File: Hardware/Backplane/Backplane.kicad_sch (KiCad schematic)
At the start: 3 parts, among them J101 10018784-10201TLF

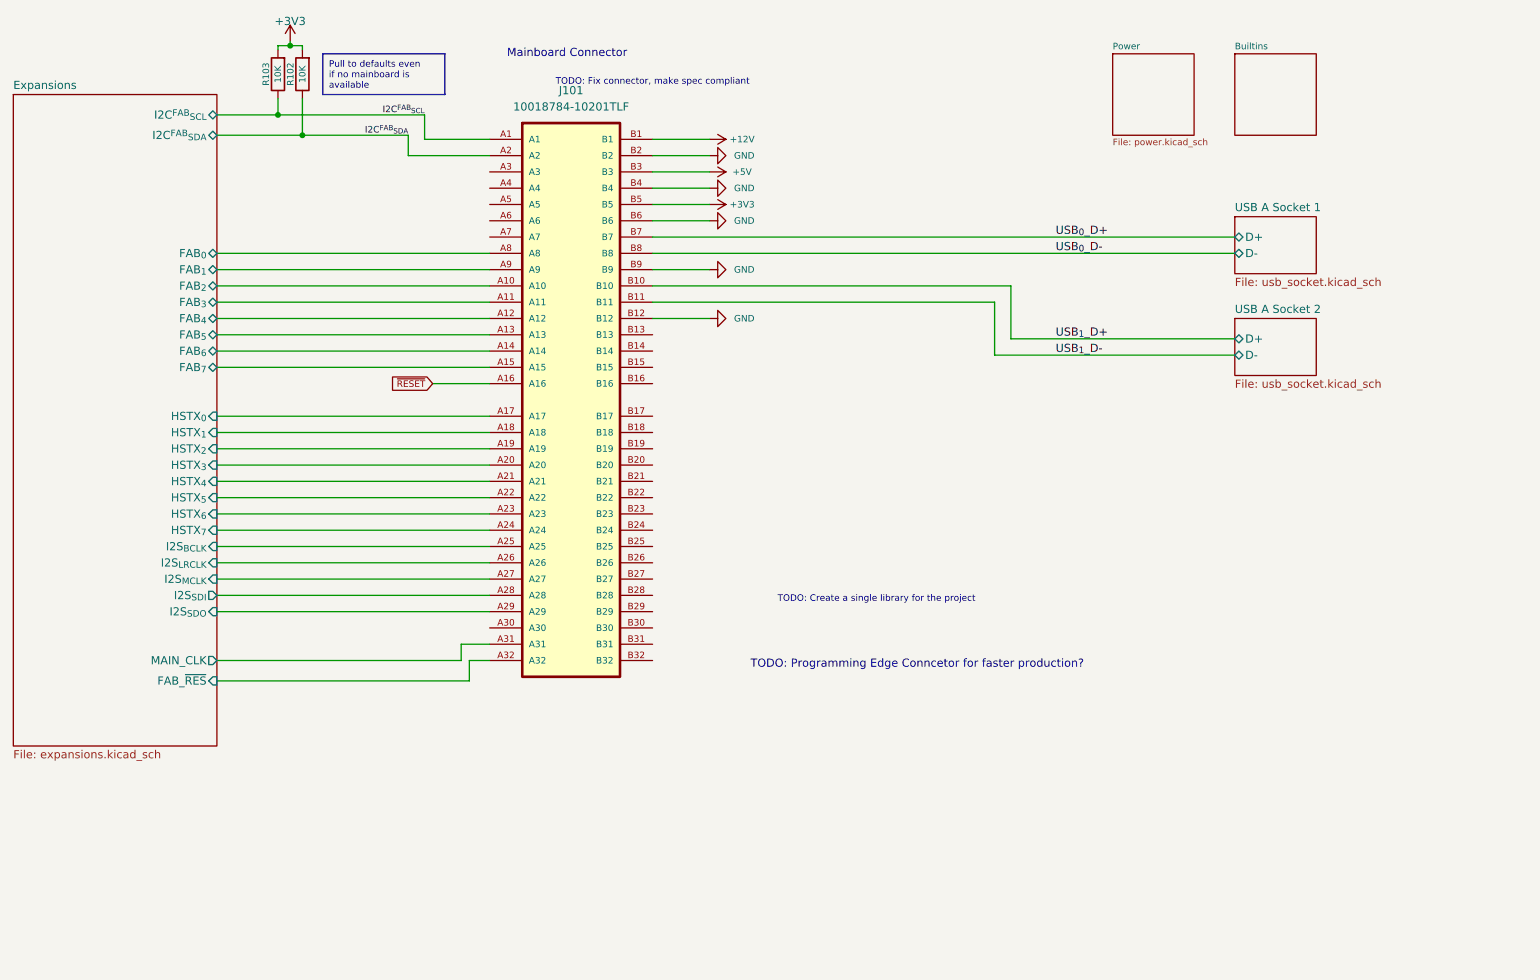
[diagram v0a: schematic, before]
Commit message: Further backplane PCB cleanup.
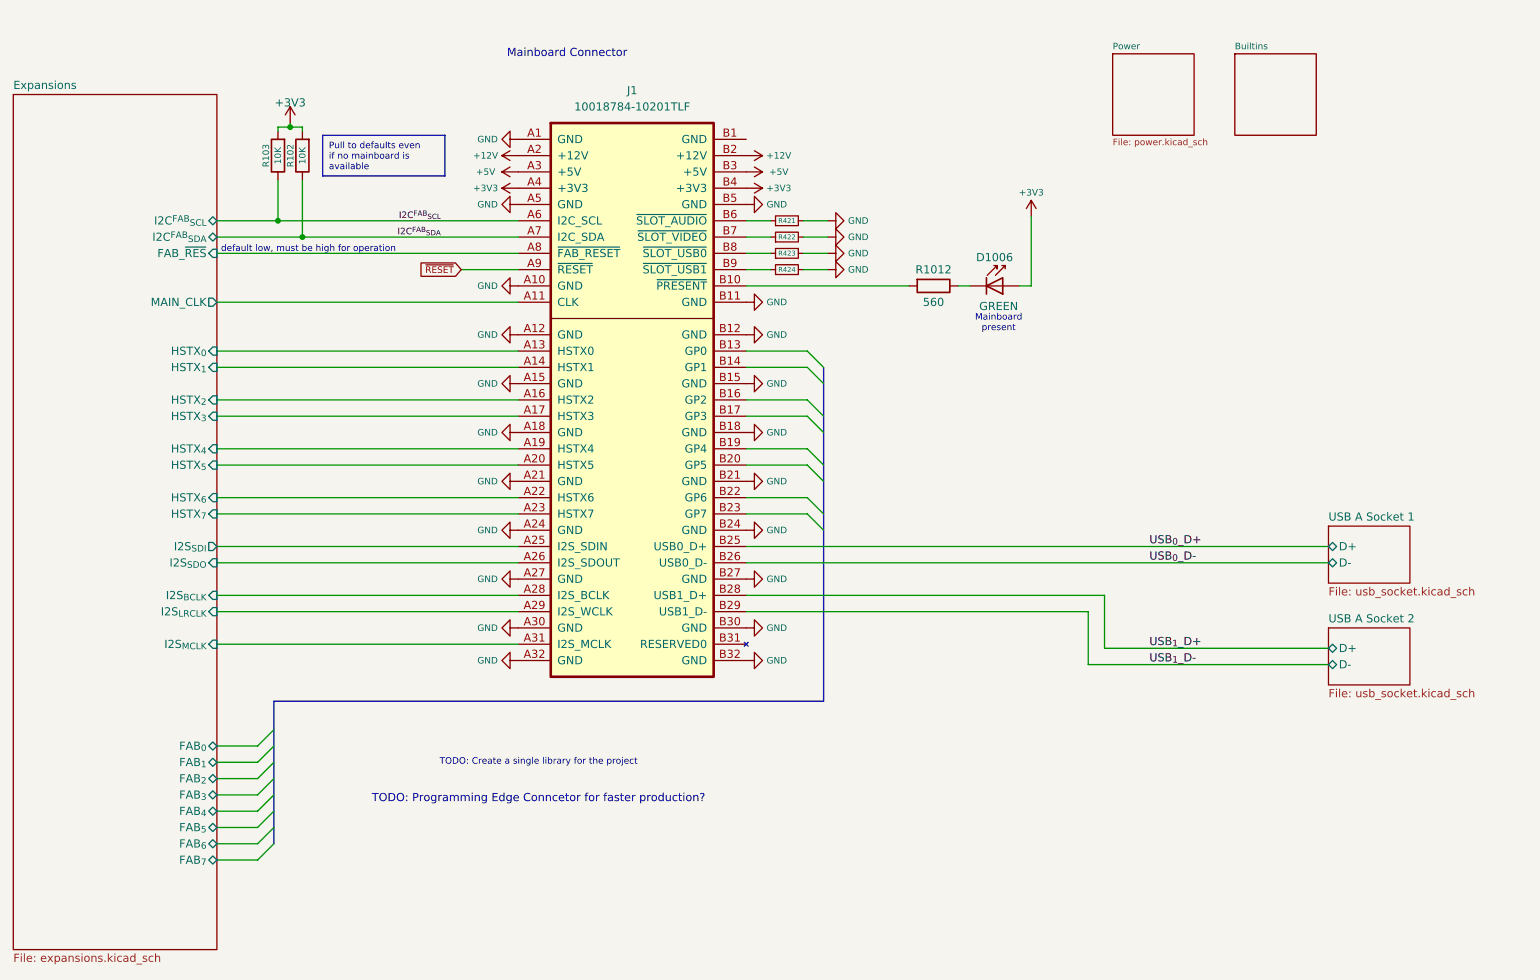
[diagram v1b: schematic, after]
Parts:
- removed J101: 10018784-10201TLF, Home Computer:CONN_10018784-10201TLF, symbol Home Computer:10018784-10201TLF
- added D1006: GREEN, LED_SMD:LED_0603_1608Metric, symbol LED:LD271
- added J1: 10018784-10201TLF, Home Computer:CONN_10018784-10201TLF, symbol Home Computer:AHC-CONN-CPU
- added R1012: 560, Resistor_SMD:R_0603_1608Metric, symbol Device:R
- added R421, R422, R423, R424: 0, Resistor_SMD:R_0603_1608Metric, symbol Device:R_Small
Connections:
- net +12V: now also J1.A2 (+12V), J1.B2 (+12V)
- net +3V3: now also D1006.2 (A), J1.A4 (+3V3), J1.B4 (+3V3)
- net +5V: now also J1.A3 (+5V), J1.B3 (+5V)
- net Expansions/FAB_~{RES}: now also J1.A8 (~{FAB_RESET})
- net Expansions/HSTX_{0}: now also J1.A13 (HSTX0)
- net Expansions/HSTX_{1}: now also J1.A14 (HSTX1)
- net Expansions/HSTX_{2}: now also J1.A16 (HSTX2)
- net Expansions/HSTX_{3}: now also J1.A17 (HSTX3)
- net Expansions/HSTX_{4}: now also J1.A19 (HSTX4)
- net Expansions/HSTX_{5}: now also J1.A20 (HSTX5)
- net Expansions/HSTX_{6}: now also J1.A22 (HSTX6)
- net Expansions/HSTX_{7}: now also J1.A23 (HSTX7)
- net Expansions/I2S_{BCLK}: now also J1.A28 (I2S_BCLK)
- net Expansions/I2S_{LRCLK}: now also J1.A29 (I2S_WCLK)
- net Expansions/I2S_{MCLK}: now also J1.A31 (I2S_MCLK)
- net Expansions/I2S_{SDI}: now also J1.A25 (I2S_SDIN)
- net Expansions/I2S_{SDO}: now also J1.A26 (I2S_SDOUT)
- net Expansions/MAIN_CLK: now also J1.A11 (CLK)
- net GND: now also J1.A1 (GND), J1.A10 (GND), J1.A12 (GND), J1.A15 (GND), J1.A18 (GND), J1.A21 (GND), J1.A24 (GND), J1.A27 (GND), J1.A30 (GND), J1.A32 (GND), J1.A5 (GND), J1.B11 (GND), J1.B12 (GND), J1.B15 (GND), J1.B18 (GND), J1.B21 (GND), J1.B24 (GND), J1.B27 (GND), J1.B30 (GND), J1.B32 (GND), J1.B5 (GND), R421.2, R422.2, R423.2, R424.2
- net I2C^{FAB}_{SCL}: now also J1.A6 (I2C_SCL)
- net I2C^{FAB}_{SDA}: now also J1.A7 (I2C_SDA)
- net USB_{0}_D+: now also J1.B25 (USB0_D+)
- net USB_{0}_D-: now also J1.B26 (USB0_D-)
- net USB_{1}_D+: now also J1.B28 (USB1_D+)
- net USB_{1}_D-: now also J1.B29 (USB1_D-)
- net ~{RESET}: now also J1.A9 (~{RESET})
- new net: J1.B10 (~{PRESENT}), R1012.2
- new net: J1.B6 (~{SLOT_AUDIO}), R421.1
- new net: J1.B7 (~{SLOT_VIDEO}), R422.1
- new net: J1.B8 (~{SLOT_USB0}), R423.1
- new net: J1.B9 (~{SLOT_USB1}), R424.1
- new net: D1006.1 (K), R1012.1
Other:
- note added: "Mainboard present"
- note added: "default low, must be high for operation"
- note removed: "TODO: Fix connector, make spec compliant"
- moved on the sheet: R102, R103
